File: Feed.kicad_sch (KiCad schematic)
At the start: 36 parts

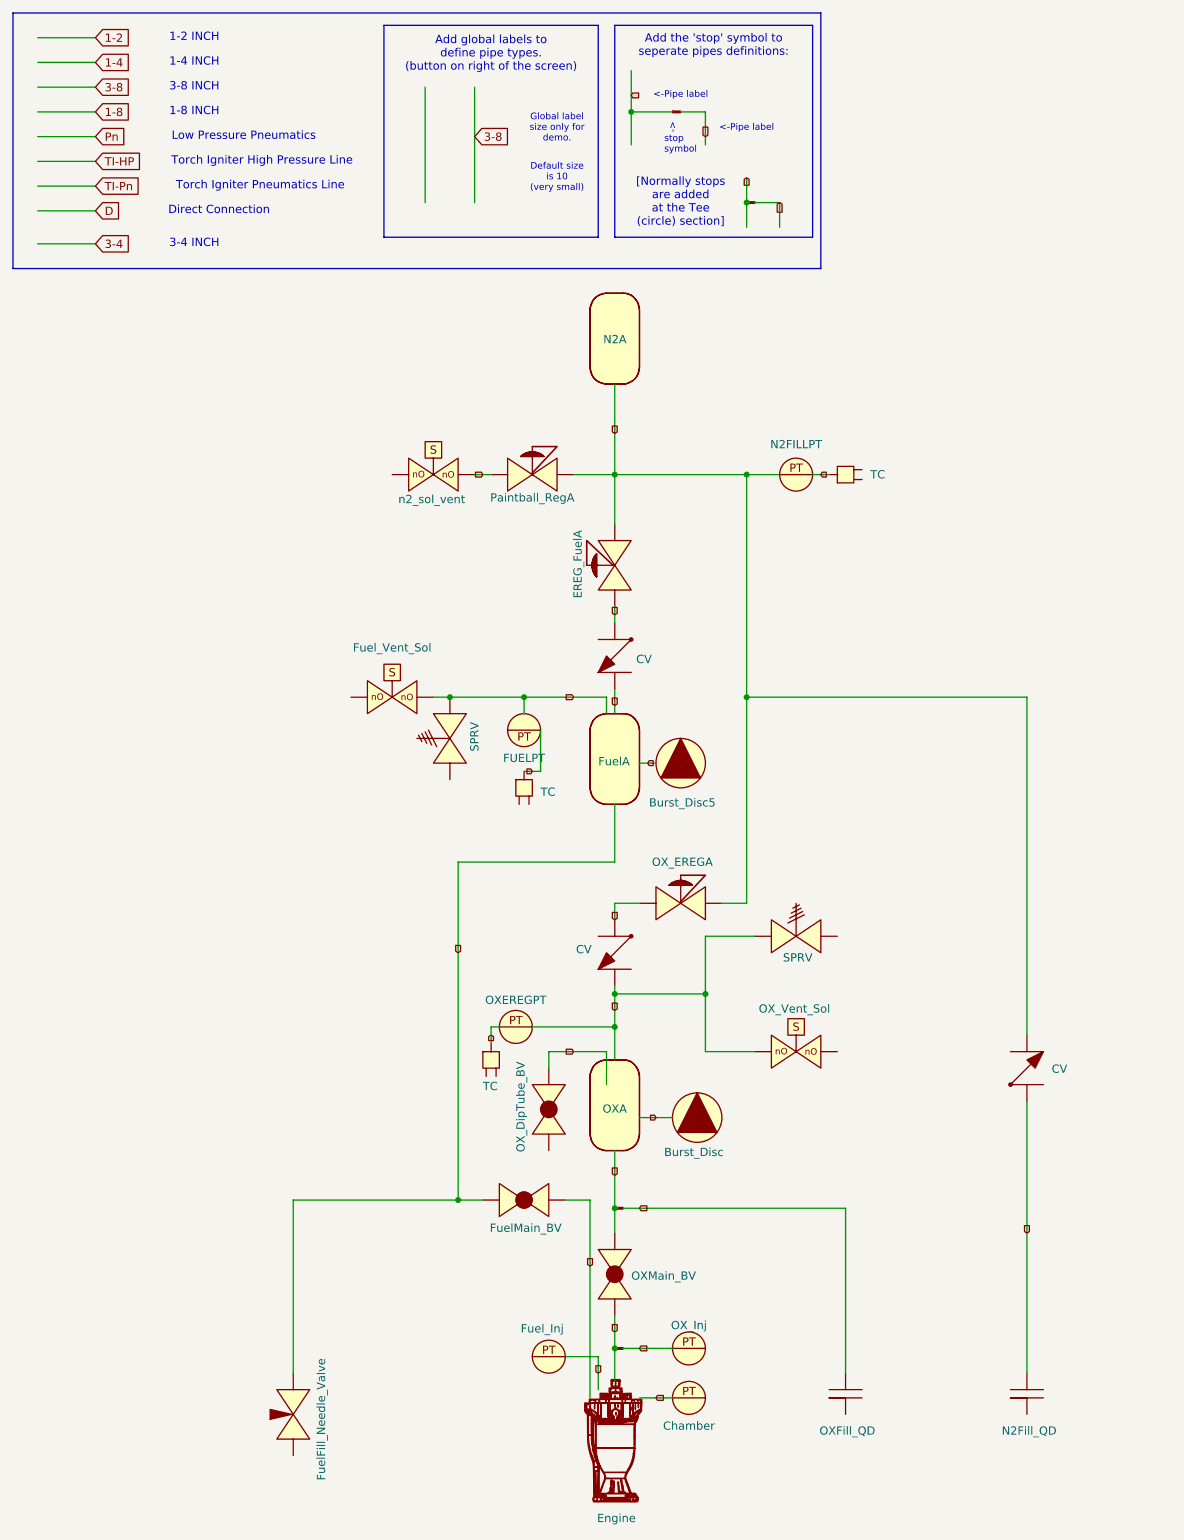
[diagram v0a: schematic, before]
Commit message: clean pnid
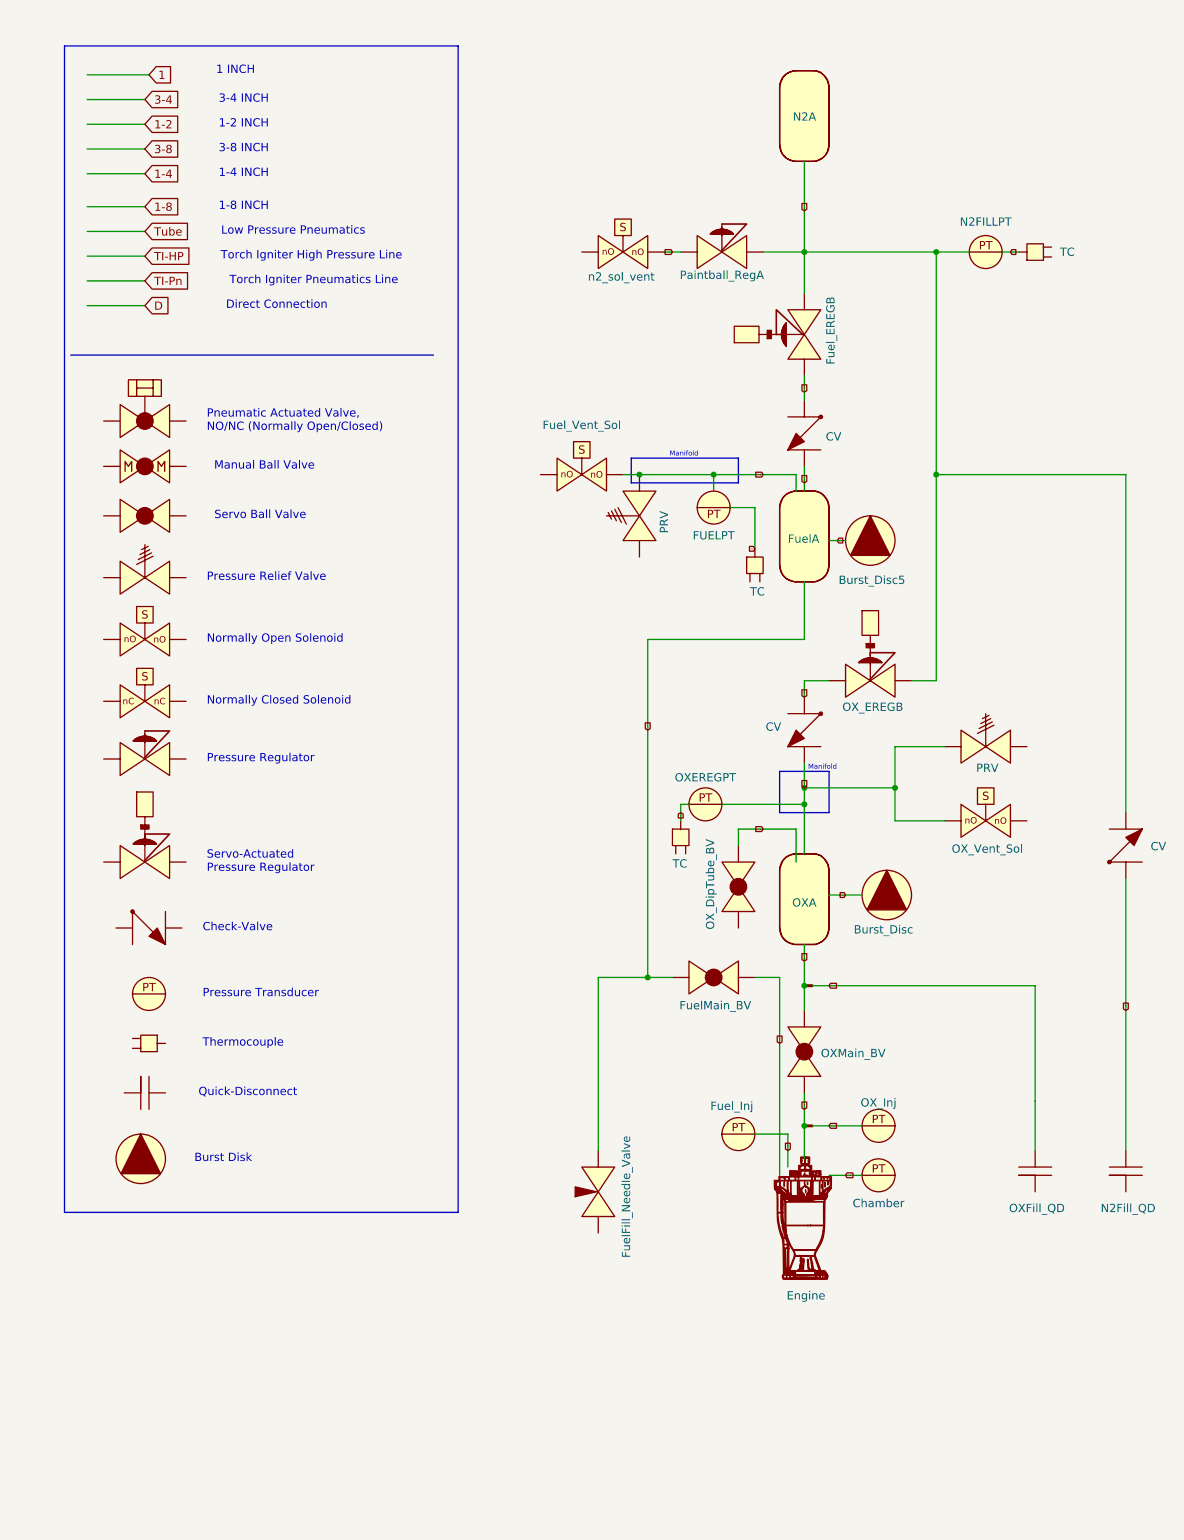
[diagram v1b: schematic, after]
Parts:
- removed EREG_Fuel, OX_EREG: ~, symbol PID_symbols:Pressure_Regulator
- removed U38, U39: ~, symbol PID_symbols:stop
- added BV45: ~, symbol PID_symbols:Ball_Valve
- added Burst_Disc6: ~, symbol PID_symbols:Burst_Disc
- added CV16: ~, symbol PID_symbols:Check_Valve
- added Fuel_EREG, OX_EREG, Servo_Reg23, Servo_Reg9: ~, symbol PID_symbols:Pressure_Regulator
- added MB_V1: ~, symbol PID_symbols:MBallValve
- added PT24: ~, symbol PID_symbols:Pressure_Transducer
- added Pmatic_B_Valve17: ~, symbol PID_symbols:Pneumatic_Rotary_Ball_Valve
- added QD30: ~, symbol PID_symbols:Quick_Disconnect
- added SPRV11: ~, symbol PID_symbols:SPRV
- added TC15: ~, symbol PID_symbols:Thermocouple
- added nC_Sol14: ~, symbol PID_symbols:Normally_Closed_Solenoid
- added nO_Sol32: ~, symbol PID_symbols:Normally Open Solenoid
- renumbered SPRV to PRV
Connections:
- net 1-4: now also Fuel_EREG., OX_EREG.
- net 3-8: now also Fuel_EREG., OX_EREG.
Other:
- note added: "1 INCH"
- note added: "Burst Disk"
- note added: "Check-Valve"
- note added: "Manifold"
- note added: "Manual Ball Valve"
- note added: "Normally Closed Solenoid"
- note added: "Normally Open Solenoid"
- note added: "Pneumatic Actuated Valve, NO/NC (Normally Open/Closed)"
- note added: "Pressure Regulator"
- note added: "Pressure Relief Valve"
- note added: "Pressure Transducer"
- note added: "Quick-Disconnect"
- note added: "Servo Ball Valve"
- note added: "Servo-Actuated Pressure Regulator"
- note added: "Thermocouple"
- note removed: "->"
- note removed: "<-Pipe label"
- note removed: "Add global labels to define pipe types. (button on right of the screen)"
- note removed: "Add the 'stop' symbol to seperate pipes definitions:"
- note removed: "Default size is 10 (very small)"
- note removed: "Global label size only for demo."
- note removed: "[Normally stops are added at the Tee (circle) section]"
- note removed: "stop symbol"
- moved on the sheet: Burst_Disc, Burst_Disc5, CV, Chamber, Engine, FUELPT, FuelA, FuelFill_Needle_Valve, FuelMain_BV, Fuel_Inj, Fuel_Vent_Sol, N2A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
